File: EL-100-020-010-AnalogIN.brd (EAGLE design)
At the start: 54 x 29.5 mm, 44 parts, among them U1 OPA2170AID, U16 24AA256-I/SN, U6 OPA2170AID, X1 9012-26, X2 944-12-08-00

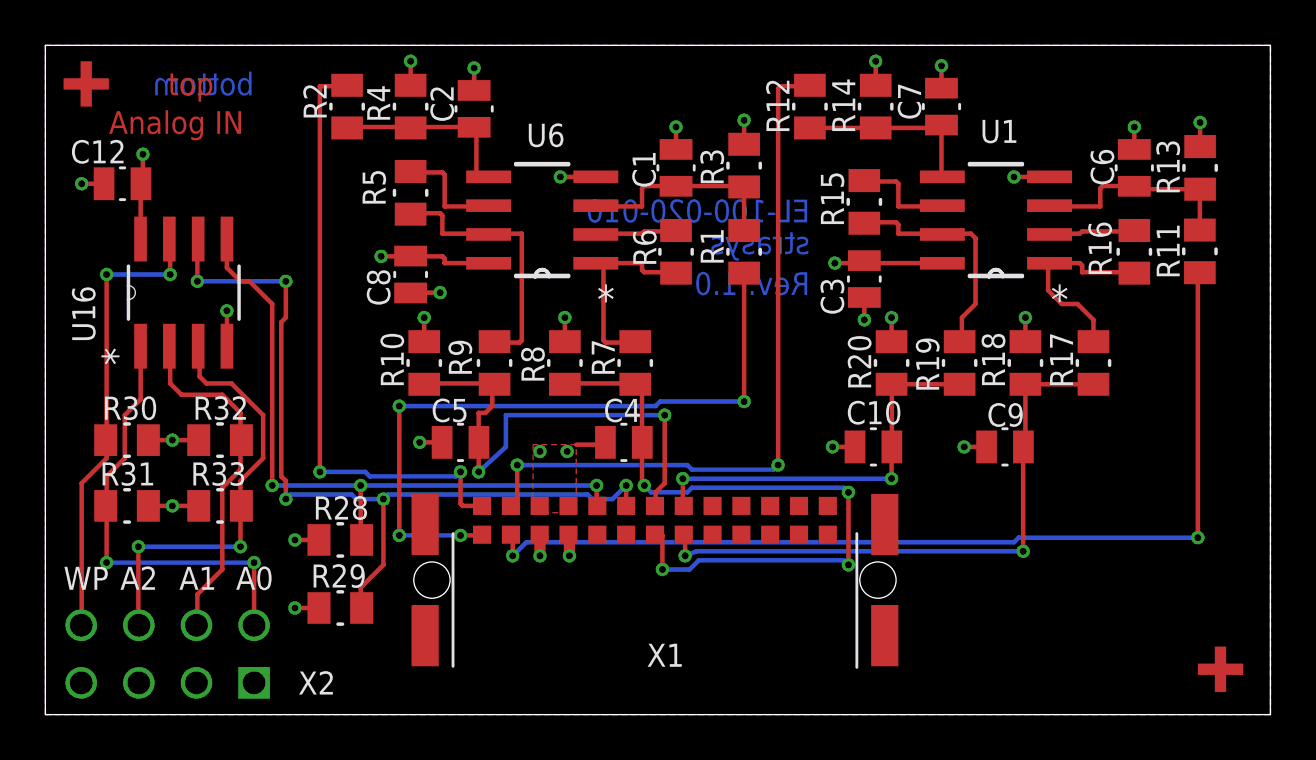
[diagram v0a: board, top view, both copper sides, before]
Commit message: DIN-Rail-production
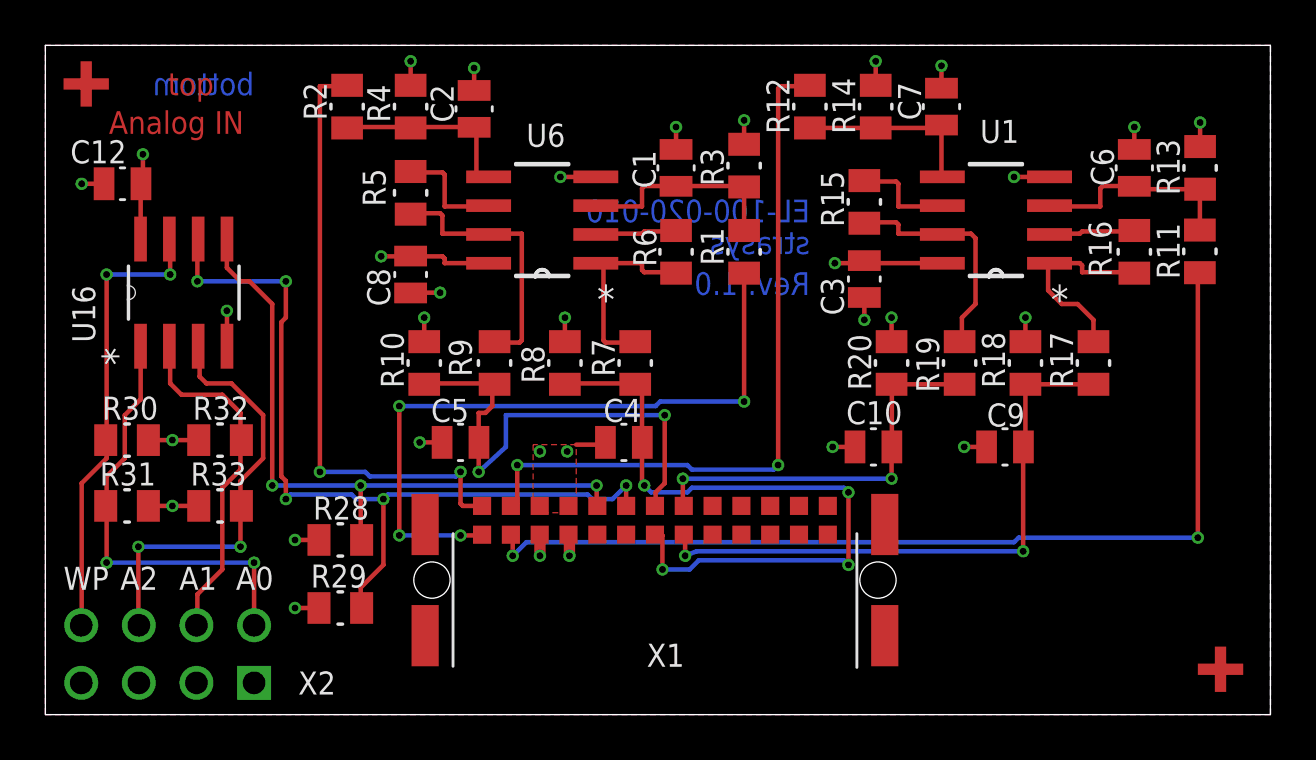
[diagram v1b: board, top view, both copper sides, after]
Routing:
- added copper zone on layer 15, net PE
